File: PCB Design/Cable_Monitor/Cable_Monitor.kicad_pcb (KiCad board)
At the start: 2 copper layers, 63.5 x 118.1 mm, 59 parts, among them J1 USB_B_Mini, P1 type="R" model="Conn_01x32_Fe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, P2 type="R" model="Conn_01x32_Fe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, Q1 BSS316N, SW1 type="R" model="SW_Push" lib=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, U1 MCP6002-xSN, U2 MCP6002-xSN, U3 SiP32508, U4 LD1117S33TR_SOT223, U5 type="R" model="DRV5053_SMD" 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, U6 type="R" model="DRV5053_THT" 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, U7 MCP6002-xSN, Y1 OpenLog, Y2 Radar K-LC5-RFB-00C

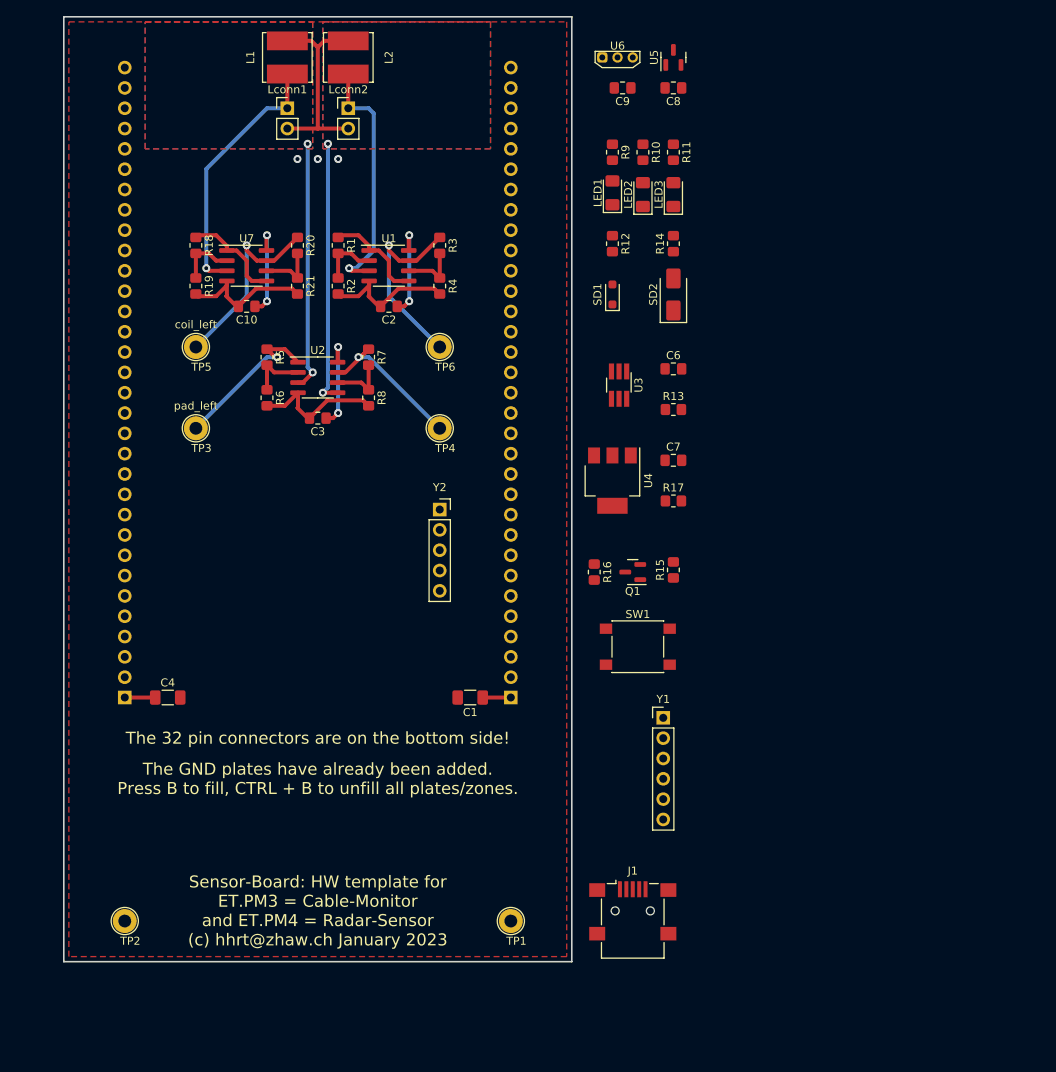
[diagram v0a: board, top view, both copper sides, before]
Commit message: PCB Layout Update
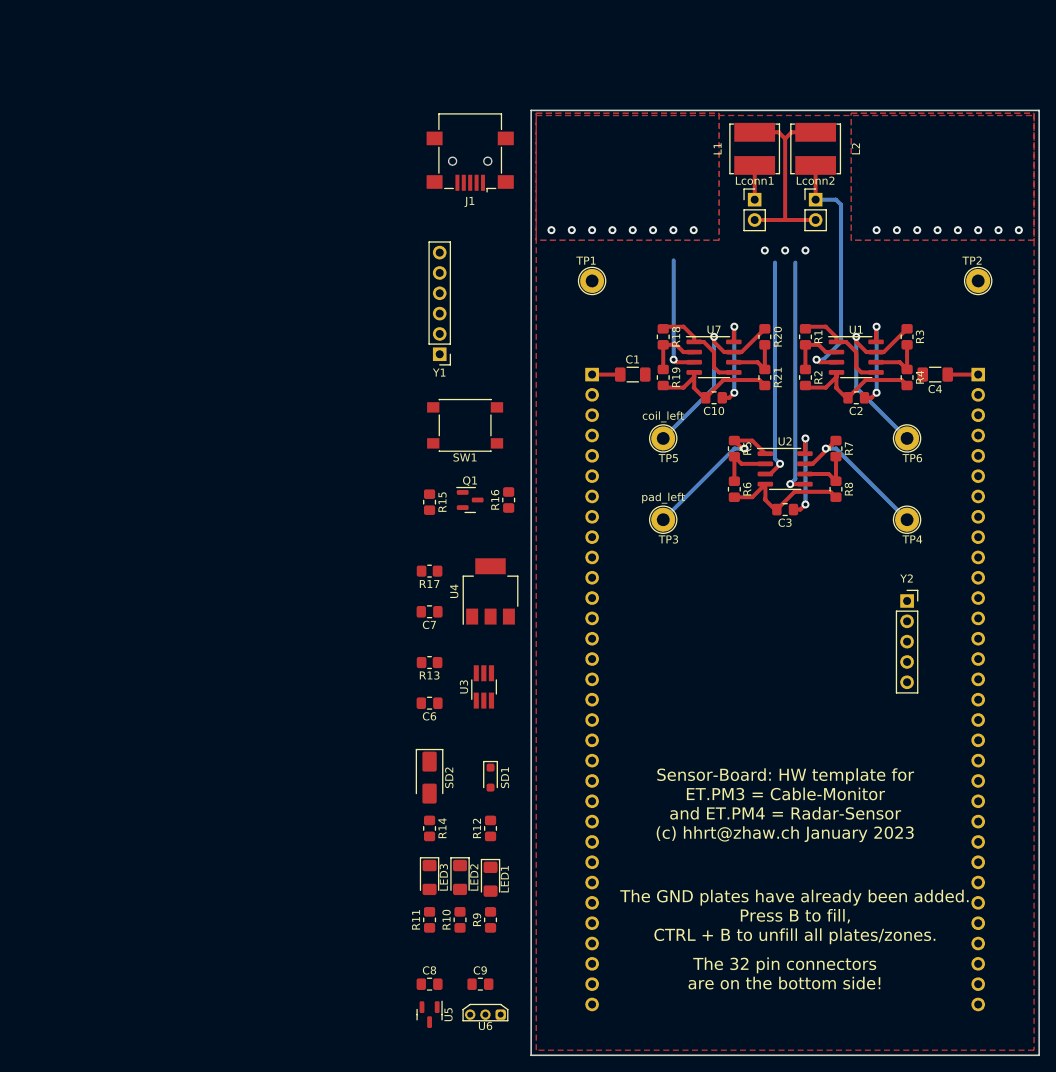
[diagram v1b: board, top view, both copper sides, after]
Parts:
- moved TP2 133.4 mm to (160.0, 54.6), turned to 180 degrees
- moved U5 123.5 mm to (91.4, 146.3), turned to -90 degrees
- moved U6 120.5 mm to (99.7, 146.3), turned to 180 degrees
- moved C8 116.1 mm to (91.4, 142.5), turned to 0 degrees
- moved P1 114.1 mm to (160.0, 66.3), turned to 180 degrees
- moved C9 113.4 mm to (97.8, 142.5), turned to 0 degrees
- moved C4 104.1 mm to (154.6, 66.3), turned to 180 degrees
- moved R11 100.7 mm to (91.4, 134.5), turned to 90 degrees
- moved R10 98.6 mm to (95.2, 134.5), turned to 90 degrees
- moved R9 97.2 mm to (99.1, 134.5), turned to 90 degrees
- moved J1 95.9 mm to (96.5, 39.6), turned to 180 degrees
- moved LED3 90.6 mm to (91.4, 129.2), turned to -90 degrees
- moved LED2 88.4 mm to (95.2, 129.2), turned to -90 degrees
- moved LED1 87.1 mm to (99.1, 129.4), turned to -90 degrees
- moved TP1 80.7 mm to (111.8, 54.6), turned to 180 degrees
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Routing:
- net coil_left: track 32.7 -> 19.4 mm
- net pad_left: track 31.2 -> 27.8 mm, vias 2 -> 9
- net pad_right: track 33.2 -> 29.8 mm, vias 2 -> 9
